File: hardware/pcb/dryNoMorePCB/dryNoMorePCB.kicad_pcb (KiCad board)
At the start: 2 copper layers, 76.2 x 44.2 mm, 34 parts, among them J1 USB_A_Stacked, J10 Barrel_Jack_MountingPin, J11 Conn_01x03, J12 Conn_01x03, J13 Conn_02x06_Odd_Even, J2 Conn_01x03, J3 Conn_01x03, J4 Conn_01x03, J5 USB_A_Stacked, J6 Conn_01x03, J7 Conn_01x03, J8 Conn_01x03, J9 USB_A_Stacked, Q1 Q_NMOS_GDSD, Q2 Q_NMOS_GDSD, Q3 Q_NMOS_GDSD, Q4 Q_NMOS_GDSD, Q5 Q_NMOS_GDSD, Q6 Q_NMOS_GDSD, U1 74HC595, U2 74HC595

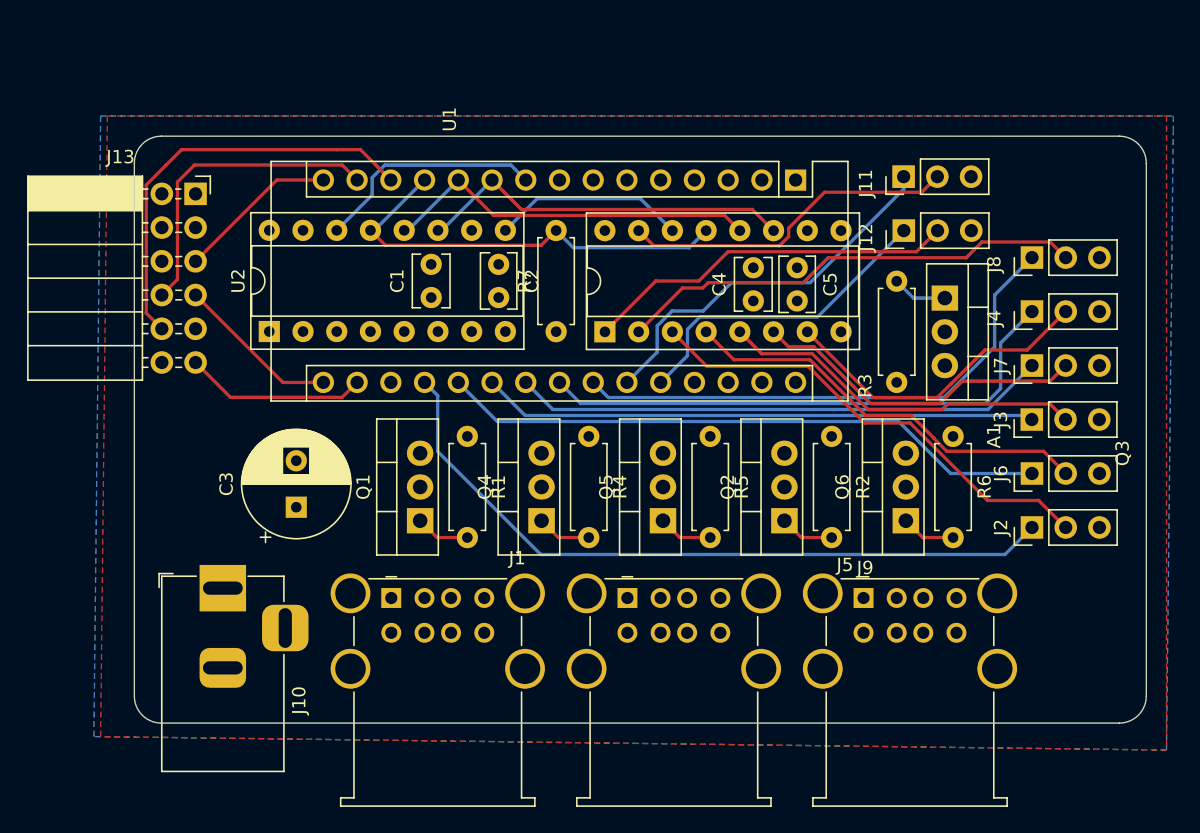
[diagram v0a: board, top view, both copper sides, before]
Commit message: more routing nightmares incoming
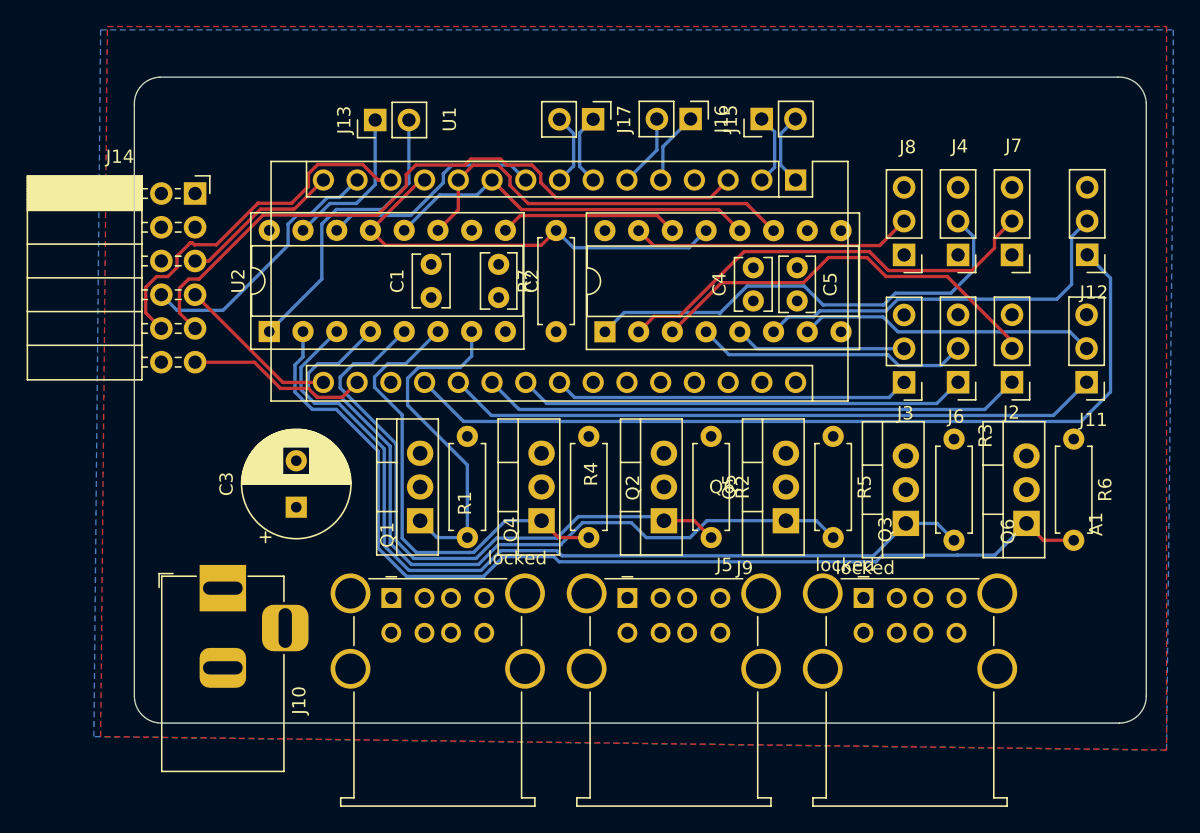
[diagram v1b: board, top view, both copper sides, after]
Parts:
- added J14: Conn_02x06_Odd_Even, Connector_PinSocket_2.54mm:PinSocket_2x06_P2.54mm_Horizontal, F.Cu at (77.7, 87.1)
- added J15: Conn_01x02, Connector_PinHeader_2.54mm:PinHeader_1x02_P2.54mm_Vertical, F.Cu at (120.4, 81.5)
- added J16: Conn_01x02, Connector_PinHeader_2.54mm:PinHeader_1x02_P2.54mm_Vertical, F.Cu at (115.0, 81.5)
- added J17: Conn_01x02, Connector_PinHeader_2.54mm:PinHeader_1x02_P2.54mm_Vertical, F.Cu at (107.7, 81.5)
- J13: value Conn_02x06_Odd_Even -> Conn_01x02; footprint Connector_PinSocket_2.54mm:PinSocket_2x06_P2.54mm_Horizontal -> Connector_PinHeader_2.54mm:PinHeader_1x02_P2.54mm_Vertical
- moved J11 20.7 mm to (144.9, 101.3), turned to 180 degrees
- moved Q3 17.2 mm to (131.2, 112.0), turned to 90 degrees
- moved J13 14.6 mm to (91.3, 81.6), turned to 90 degrees
- moved J12 13.9 mm to (144.9, 91.7), turned to 180 degrees
- moved J2 11.0 mm to (139.2, 101.3), turned to 180 degrees
- moved J3 10.0 mm to (131.1, 101.3), turned to 180 degrees
- moved J8 9.63 mm to (131.1, 91.7), turned to 180 degrees
- moved Q5 9.26 mm to (122.2, 111.8)
- moved R5 9.26 mm to (125.8, 105.4)
- moved Q6 9.09 mm to (140.3, 112.0)
- moved R6 9.09 mm to (143.9, 105.6)
- moved R2 9.07 mm to (116.6, 105.4)
- moved Q2 9.07 mm to (113.0, 111.8)
- moved J6 8.84 mm to (135.2, 101.3), turned to 180 degrees
- moved J7 8.47 mm to (139.2, 91.7), turned to 180 degrees
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- renumbered J1 to locked, J9 to locked, J5 to locked
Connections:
- A1 pad 1: unconnected-(A1-Pad1) -> /UNUSED_D_PIN_2
- A1 pad 10: /PWR_CTRL_SHIFT_REG_IN_CLK -> /PWR_CTRL_SHIFT_REG_UPDATE
- A1 pad 11: /PWR_CTRL_SHIFT_REG_UPDATE -> /PWR_CTRL_SHIFT_REG_IN_CLK
- A1 pad 19: /MOIST_SENS_AOUT_1 -> /WAT_LVL_SENS_AOUT_2
- A1 pad 2: unconnected-(A1-Pad2) -> /UNUSED_D_PIN_1
- A1 pad 20: /MOIST_SENS_AOUT_2 -> /WAT_LVL_SENS_AOUT_1
- A1 pad 21: /MOIST_SENS_AOUT_3 -> /MOIST_SENS_AOUT_1
- A1 pad 22: /MOIST_SENS_AOUT_4 -> /MOIST_SENS_AOUT_2
- A1 pad 23: /MOIST_SENS_AOUT_5 -> /MOIST_SENS_AOUT_3
- A1 pad 25: /WAT_LVL_SENS_AOUT_1 -> /MOIST_SENS_AOUT_5
- A1 pad 26: /WAT_LVL_SENS_AOUT_2 -> /MOIST_SENS_AOUT_4
- A1 pad 28: /ETH_RST -> unconnected-(A1-Pad28)
- A1 pad 5: unconnected-(A1-Pad5) -> /UNUSED_D_PIN_3
- A1 pad 6: unconnected-(A1-Pad6) -> /UNUSED_D_PIN_4
- A1 pad 7: unconnected-(A1-Pad7) -> /UNUSED_D_PIN_5
- A1 pad 8: unconnected-(A1-Pad8) -> /UNUSED_D_PIN_6
- J13 pad 1: +5V -> /UNUSED_PWR_CTRL_1
- J13 pad 2: GND -> /UNUSED_PWR_CTRL_2
- U1 pad 1: /WAT_LVL_SENS_PWR_2 -> /MOIST_SENS_PWR_5
- U1 pad 15: /WAT_LVL_SENS_PWR_1 -> /MOIST_SENS_PWR_6
- U1 pad 2: /MOIST_SENS_PWR_6 -> /MOIST_SENS_PWR_4
- U1 pad 6: /MOIST_SENS_PWR_4 -> /WAT_LVL_SENS_PWR_2
- U1 pad 7: /MOIST_SENS_PWR_5 -> /WAT_LVL_SENS_PWR_1
- U2 pad 1: /PUMP_2_CTRL -> /UNUSED_PWR_CTRL_2
- U2 pad 15: /PUMP_1_CTRL -> /UNUSED_PWR_CTRL_1
- U2 pad 2: /PUMP_3_CTRL -> /PUMP_6_CTRL
- U2 pad 3: /PUMP_4_CTRL -> /PUMP_5_CTRL
- U2 pad 4: /PUMP_5_CTRL -> /PUMP_4_CTRL
- U2 pad 5: /PUMP_6_CTRL -> /PUMP_3_CTRL
- U2 pad 6: unconnected-(U2-Pad6) -> /PUMP_2_CTRL
- U2 pad 7: unconnected-(U2-Pad7) -> /PUMP_1_CTRL
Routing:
- net /PUMP_6_CTRL: track 4.08 -> 76.0 mm
- net /PUMP_5_CTRL: track 4.15 -> 66.9 mm
- net /PUMP_4_CTRL: track 4.08 -> 59.3 mm
- net /ETH_RST: track 0.00 -> 51.5 mm
- net /PUMP_3_CTRL: track 4.08 -> 46.5 mm
- net /MOIST_SENS_AOUT_5: track 41.1 -> 0.00 mm
- net /WAT_LVL_SENS_AOUT_2: track 24.2 -> 64.8 mm
- net /MOIST_SENS_AOUT_4: track 40.3 -> 0.00 mm
- net /MOIST_SENS_AOUT_6: track 40.2 -> 0.00 mm
- net /PUMP_2_CTRL: track 4.08 -> 35.2 mm
- net /UNUSED_PWR_CTRL_2: track 0.00 -> 22.3 mm
- net /PUMP_1_CTRL: track 4.08 -> 25.3 mm
- net /WAT_LVL_SENS_AOUT_1: track 30.1 -> 49.4 mm
- net /MOIST_SENS_AOUT_3: track 41.8 -> 26.9 mm
- net /MOIST_SENS_PWR_3: track 27.6 -> 12.9 mm
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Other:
- board size 76.2 x 44.2 mm -> 76.2 x 48.6 mm
- board text added: "J5"
- board text added: "J9"
- board text added: "Q6"

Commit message: almost done with the pcb
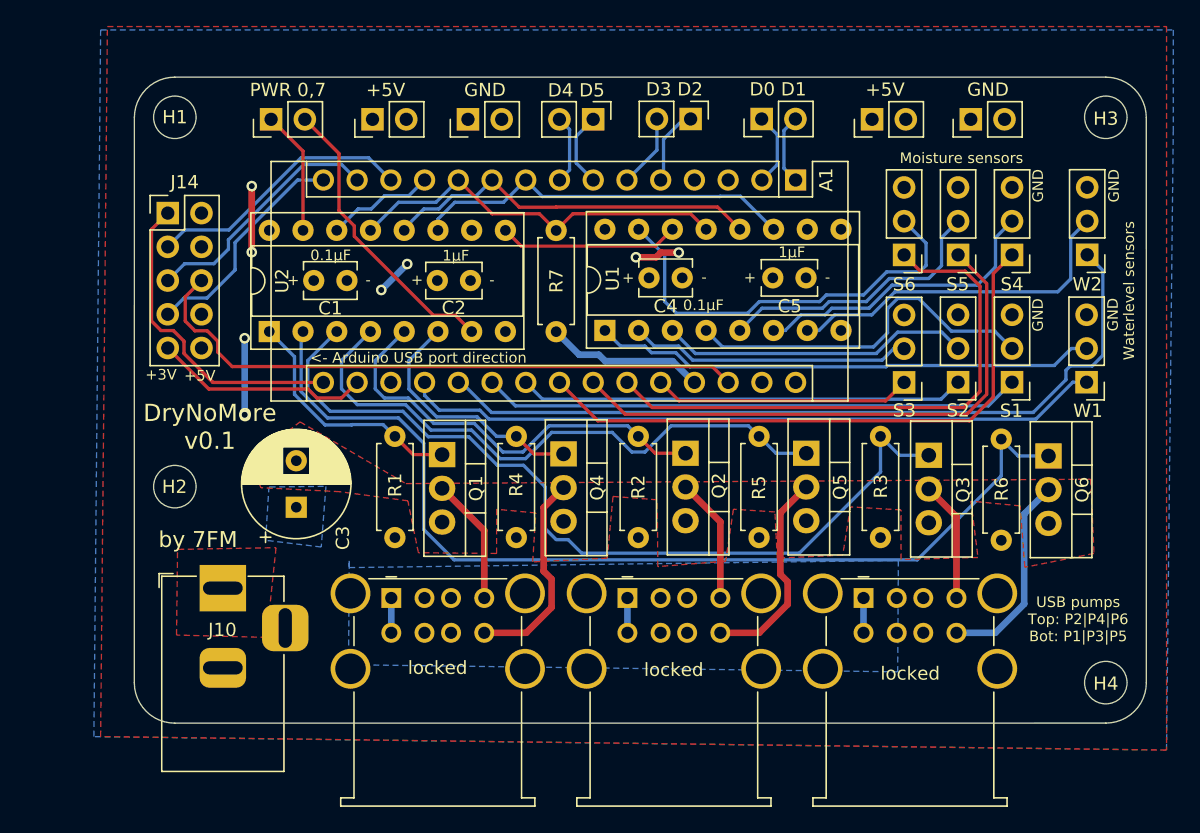
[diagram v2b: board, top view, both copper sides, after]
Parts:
- added +5V: +5V, Connector_PinHeader_2.54mm:PinHeader_1x02_P2.54mm_Vertical, F.Cu at (91.1, 81.5)
- added +5V: +5V, Connector_PinHeader_2.54mm:PinHeader_1x02_P2.54mm_Vertical, F.Cu at (128.7, 81.5)
- added GND: GND, Connector_PinHeader_2.54mm:PinHeader_1x02_P2.54mm_Vertical, F.Cu at (98.3, 81.5)
- added GND: GND, Connector_PinHeader_2.54mm:PinHeader_1x02_P2.54mm_Vertical, F.Cu at (136.1, 81.5)
- added H1: MountingHole, MountingHole:MountingHole_3.2mm_M3_DIN965, F.Cu at (76.2, 81.4)
- added H2: MountingHole, MountingHole:MountingHole_3.2mm_M3_DIN965, F.Cu at (76.2, 109.2)
- added H3: MountingHole, MountingHole:MountingHole_3.2mm_M3_DIN965, F.Cu at (146.3, 81.4)
- added H4: MountingHole, MountingHole:MountingHole_3.2mm_M3_DIN965, F.Cu at (146.3, 124.0)
- D0 D1: renamed from J15
- D3 D2: renamed from J16
- D4 D5: renamed from J17
- J14: value Conn_02x06_Odd_Even -> ETH_W5500; footprint Connector_PinSocket_2.54mm:PinSocket_2x06_P2.54mm_Horizontal -> Connector_PinHeader_2.54mm:PinHeader_2x05_P2.54mm_Vertical
- PWR 0,7: renamed from J13
- moved R5 9.44 mm to (120.2, 113.0), turned to 90 degrees
- moved R2 9.39 mm to (111.1, 113.0), turned to 90 degrees
- moved R1 9.37 mm to (92.8, 113.0), turned to 90 degrees
- moved R4 9.37 mm to (101.9, 113.0), turned to 90 degrees
- moved R6 9.37 mm to (138.4, 113.2), turned to 90 degrees
- moved R3 9.26 mm to (129.3, 113.0), turned to 90 degrees
- moved PWR 0,7 7.84 mm to (83.4, 81.5)
- moved C1 6.47 mm to (89.2, 93.7), turned to 180 degrees
- moved C4 5.63 mm to (114.4, 93.5), turned to 180 degrees
- moved Q3 5.41 mm to (133.0, 106.8), turned to -90 degrees
- moved Q6 5.34 mm to (142.0, 106.9), turned to -90 degrees
- moved Q2 5.33 mm to (114.7, 106.7), turned to -90 degrees
- moved Q5 5.31 mm to (123.7, 106.7), turned to -90 degrees
- moved Q4 5.29 mm to (105.5, 106.7), turned to -90 degrees
- moved Q1 5.25 mm to (96.3, 106.8), turned to -90 degrees
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- renumbered J2 to S1, J6 to S2, J3 to S3, J7 to S4, J4 to S5, J8 to S6, J11 to W1, J12 to W2
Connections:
- A1 pad 11: /PWR_CTRL_SHIFT_REG_IN_CLK -> /PWR_CTRL_SHIFT_REG_OE
- A1 pad 12: /PWR_CTRL_SHIFT_REG_OE -> /PWR_CTRL
- A1 pad 19: /WAT_LVL_SENS_AOUT_2 -> /WAT_LVL_SENS_AOUT_1
- A1 pad 20: /WAT_LVL_SENS_AOUT_1 -> /WAT_LVL_SENS_AOUT_2
- A1 pad 23: /MOIST_SENS_AOUT_3 -> /MOIST_SENS_AOUT_4
- A1 pad 24: /MOIST_SENS_AOUT_6 -> /MOIST_SENS_AOUT_5
- A1 pad 25: /MOIST_SENS_AOUT_5 -> /MOIST_SENS_AOUT_6
- A1 pad 26: /MOIST_SENS_AOUT_4 -> /MOIST_SENS_AOUT_3
- A1 pad 28: unconnected-(A1-Pad28) -> /ETH_RST
- A1 pad 3: /ETH_RST -> unconnected-(A1-Pad3)
- A1 pad 9: /PWR_CTRL -> /PWR_CTRL_SHIFT_REG_IN_CLK
- J14 pad 1: +5V -> /ETH_SCLK
- J14 pad 10: /ETH_CS -> +5V
- J14 pad 2: GND -> unconnected-(J14-Pad2)
- J14 pad 3: /ETH_INT -> /ETH_CS
- J14 pad 4: /ETH_CLK_OUT -> /ETH_INT
- J14 pad 5: /ETH_MISO -> /ETH_MOSI
- J14 pad 6: /ETH_WAKE_ON_LAN -> /ETH_RST
- J14 pad 7: /ETH_SCLK -> /ETH_MISO
- J14 pad 8: /ETH_MOSI -> GND
- J14 pad 9: /ETH_RST -> +3V3
- U1 pad 1: /MOIST_SENS_PWR_5 -> /WAT_LVL_SENS_PWR_1
- U1 pad 2: /MOIST_SENS_PWR_4 -> /MOIST_SENS_PWR_3
- U1 pad 3: /MOIST_SENS_PWR_1 -> /MOIST_SENS_PWR_2
- U1 pad 4: /MOIST_SENS_PWR_2 -> /MOIST_SENS_PWR_1
- U1 pad 5: /MOIST_SENS_PWR_3 -> /MOIST_SENS_PWR_5
- U1 pad 6: /WAT_LVL_SENS_PWR_2 -> /MOIST_SENS_PWR_4
- U1 pad 7: /WAT_LVL_SENS_PWR_1 -> /WAT_LVL_SENS_PWR_2
- U2 pad 1: /UNUSED_PWR_CTRL_2 -> /PUMP_1_CTRL
- U2 pad 7: /PUMP_1_CTRL -> /UNUSED_PWR_CTRL_2
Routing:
- net /MOIST_SENS_AOUT_4: track 0.00 -> 45.9 mm
- net /MOIST_SENS_AOUT_5: track 0.00 -> 42.6 mm
- net /MOIST_SENS_AOUT_6: track 0.00 -> 42.5 mm
- net +5V: track 0.00 -> 28.1 mm, vias 0 -> 4
- net /PUMP_2_CTRL: track 35.2 -> 18.9 mm
- net /PUMP_4_PWR: track 0.00 -> 15.8 mm
- net /PUMP_2_PWR: track 0.00 -> 15.7 mm
- net /WAT_LVL_SENS_PWR_1: track 22.5 -> 38.0 mm
- net /PUMP_6_PWR: track 0.00 -> 15.4 mm
- net /PUMP_3_CTRL: track 46.5 -> 32.2 mm
- net /MOIST_SENS_PWR_5: track 35.1 -> 21.1 mm
- net /PUMP_4_CTRL: track 59.3 -> 45.5 mm
- net /ETH_SCLK: track 12.4 -> 24.0 mm
- net /MOIST_SENS_PWR_6: track 21.2 -> 31.8 mm
- net /MOIST_SENS_PWR_4: track 33.2 -> 22.7 mm
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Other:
- outline, holes or cut-outs redrawn
- board text added: "+"
- board text added: "+3V"
- board text added: "+5V"
- board text added: "-"
- board text added: "0.1µF"
- board text added: "1µF"
- board text added: "<- Arduino USB port direction"
- board text added: "C1"
- board text added: "C2"
- board text added: "C4"
- board text added: "C5"
- board text added: "DryNoMore v0.1"
- board text added: "GND"
- board text added: "Moisture sensors"
- board text added: "USB pumps Top: P2|P4|P6 Bot: P1|P3|P5"
- board text added: "Waterlevel sensors"
- board text added: "by 7FM"
- board text removed: "J5"
- board text removed: "J9"
- board text removed: "Q6"
